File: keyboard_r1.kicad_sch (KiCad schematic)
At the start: 1 part, among them U1 Pico

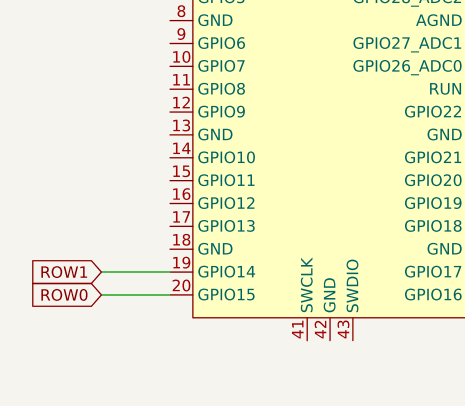
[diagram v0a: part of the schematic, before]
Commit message: added all global labels
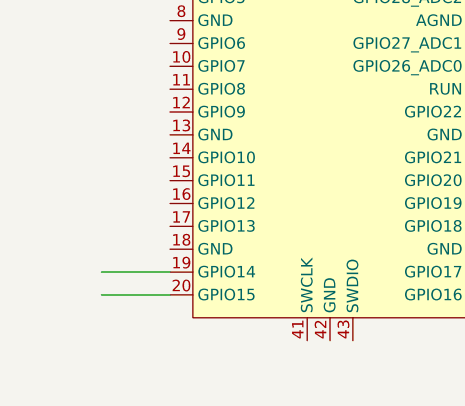
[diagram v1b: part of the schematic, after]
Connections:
- net ROW0: no longer names the net of U1.20 (GPIO15)
- net ROW1: no longer names the net of U1.19 (GPIO14)
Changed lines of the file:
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@@
     (stroke (width 0) (type default) (color 0 0 0 0))
-  )
-  (global_label "ROW1" (shape input) (at 67.31 82.55 180) (fields_autoplaced)
-    (effects (font (size 1.27 1.27)) (justify right))
-    (property "Intersheet References" "${INTERSHEET_REFS}" (id 0) (at 59.6355 82.4706 0)
-      (effects (font (size 1.27 1.27)) (justify right) hide)
-    )
-  )
-  (global_label "ROW0" (shape input) (at 67.31 85.09 180) (fields_autoplaced)
-    (effects (font (size 1.27 1.27)) (justify right))
-    (property "Intersheet References" "${INTERSHEET_REFS}" (id 0) (at 59.6355 85.0106 0)
-      (effects (font (size 1.27 1.27)) (justify right) hide)
-    )
   )
   (symbol (lib_id "MCU_RaspberryPi_and_Boards:Pico") (at 92.71 60.96 0) (unit 1)
